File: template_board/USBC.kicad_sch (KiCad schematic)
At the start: 13 parts, among them J1 USB_C_Receptacle_USB2.0_16P, U1 IP4220CZ6, U11 FSUSB42UMX, U3 IP4220CZ6

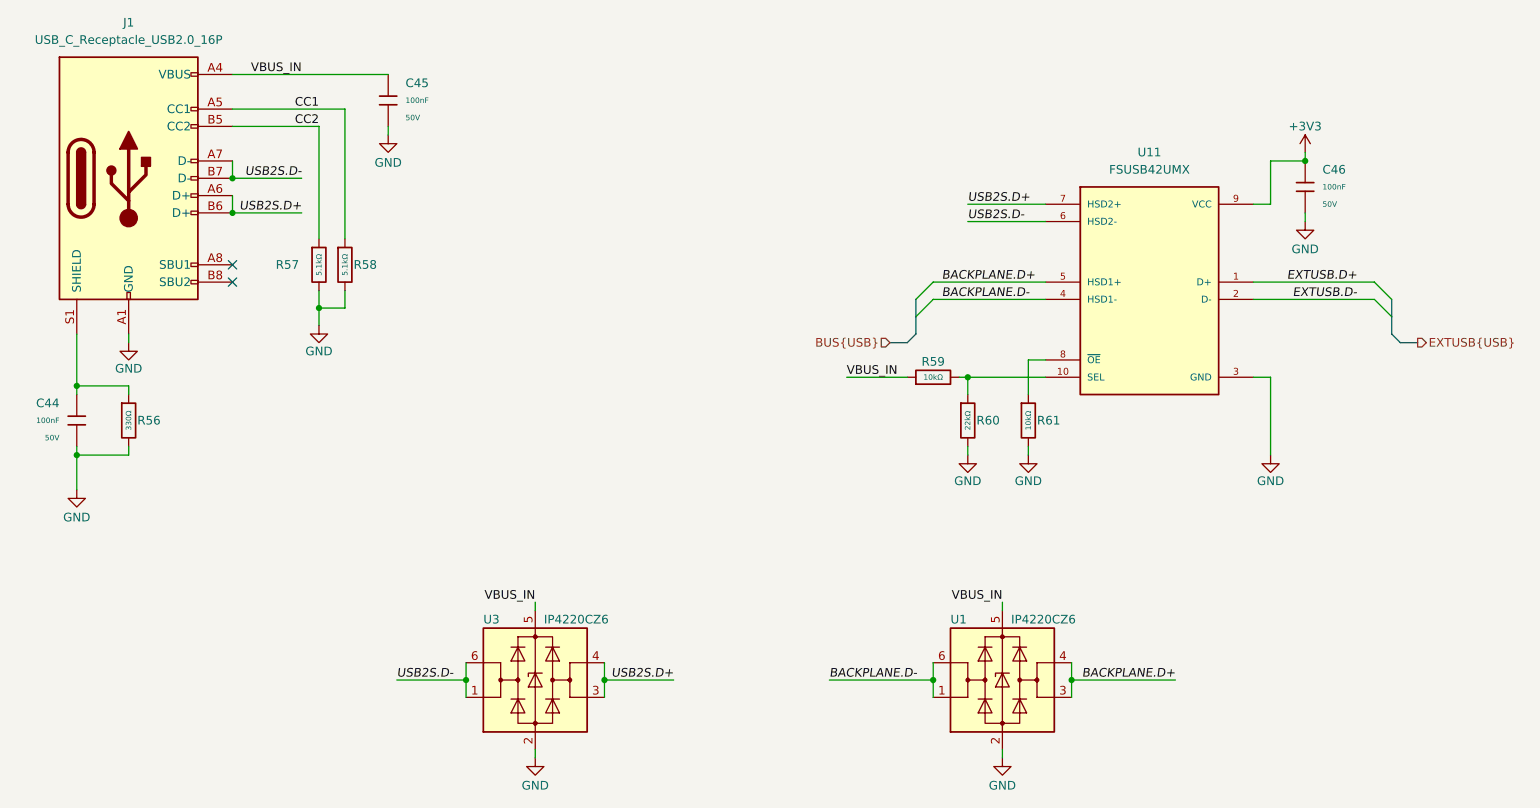
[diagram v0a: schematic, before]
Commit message: chamt skończony chyba
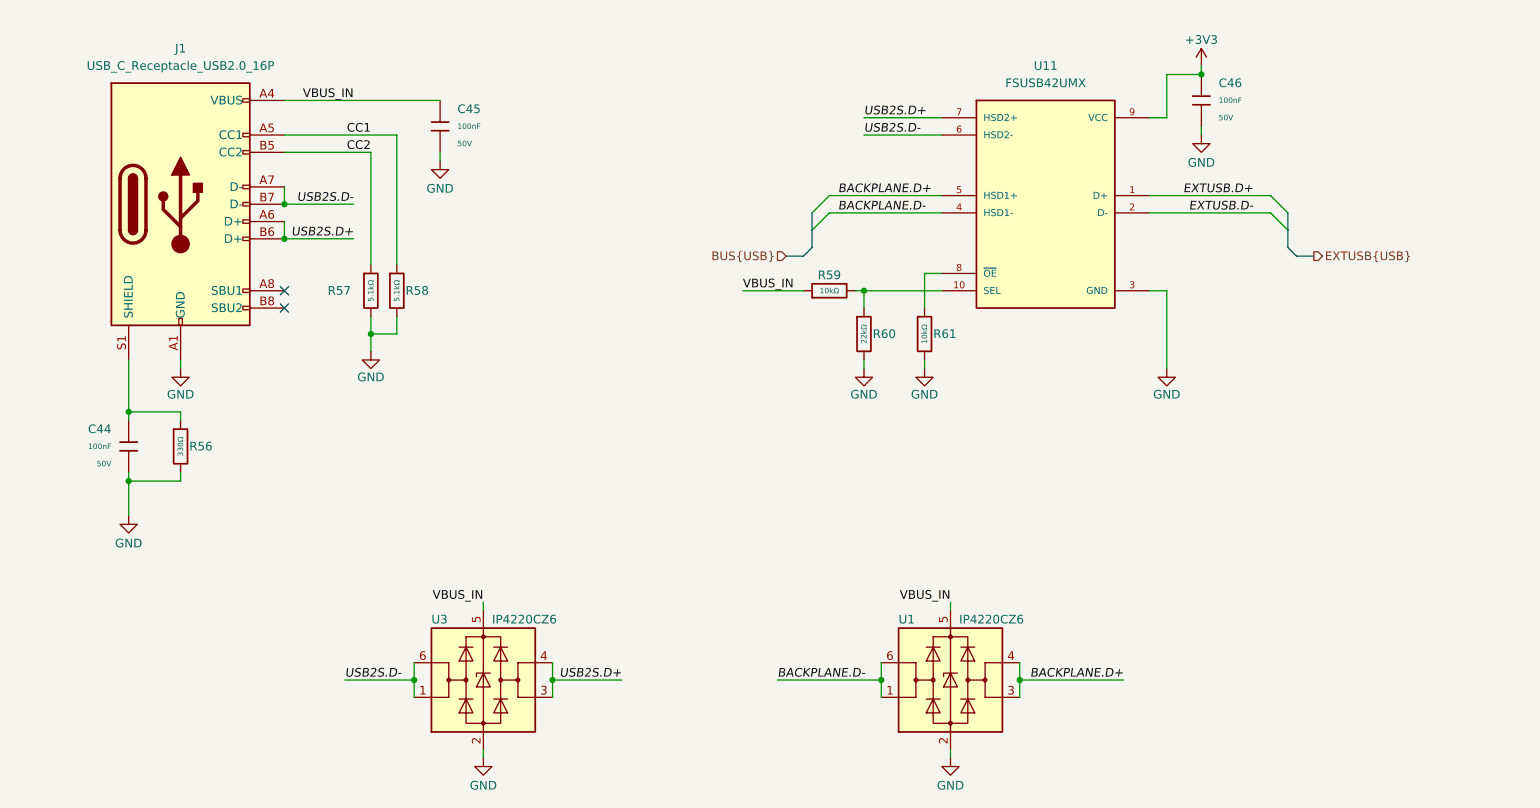
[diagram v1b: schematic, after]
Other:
- moved on the sheet: C44, C45, C46, J1, R56, R57, R58, R59, R60, R61, U1, U11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
